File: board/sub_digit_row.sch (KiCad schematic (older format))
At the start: 86 parts, among them Q601 Q_PMOS_GSD, Q602 Q_PMOS_GSD, Q603 Q_PMOS_GSD, Q604 Q_PMOS_GSD, Q605 Q_PMOS_GSD, Q606 Q_PMOS_GSD, Q607 Q_PMOS_GSD, Q608 Q_PMOS_GSD, U601 TPIC6D595, U602 TPIC6D595, U603 TPIC6D595

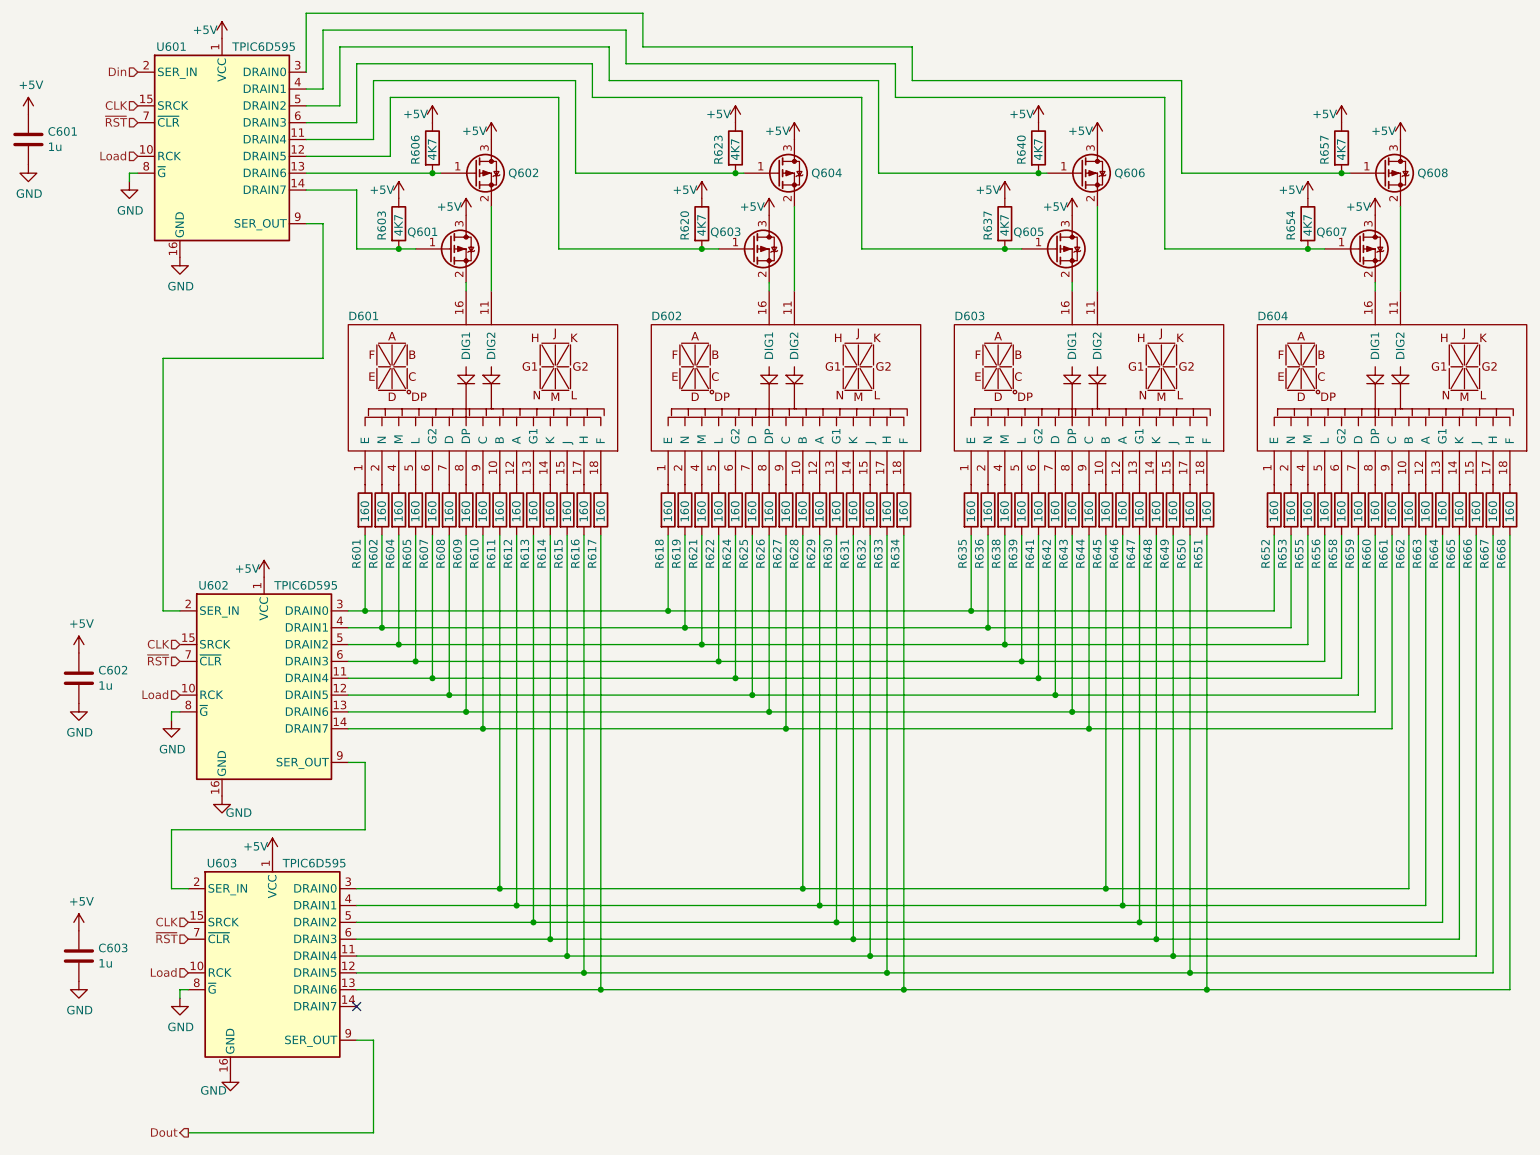
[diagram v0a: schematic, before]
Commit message: Schematics mostly complete
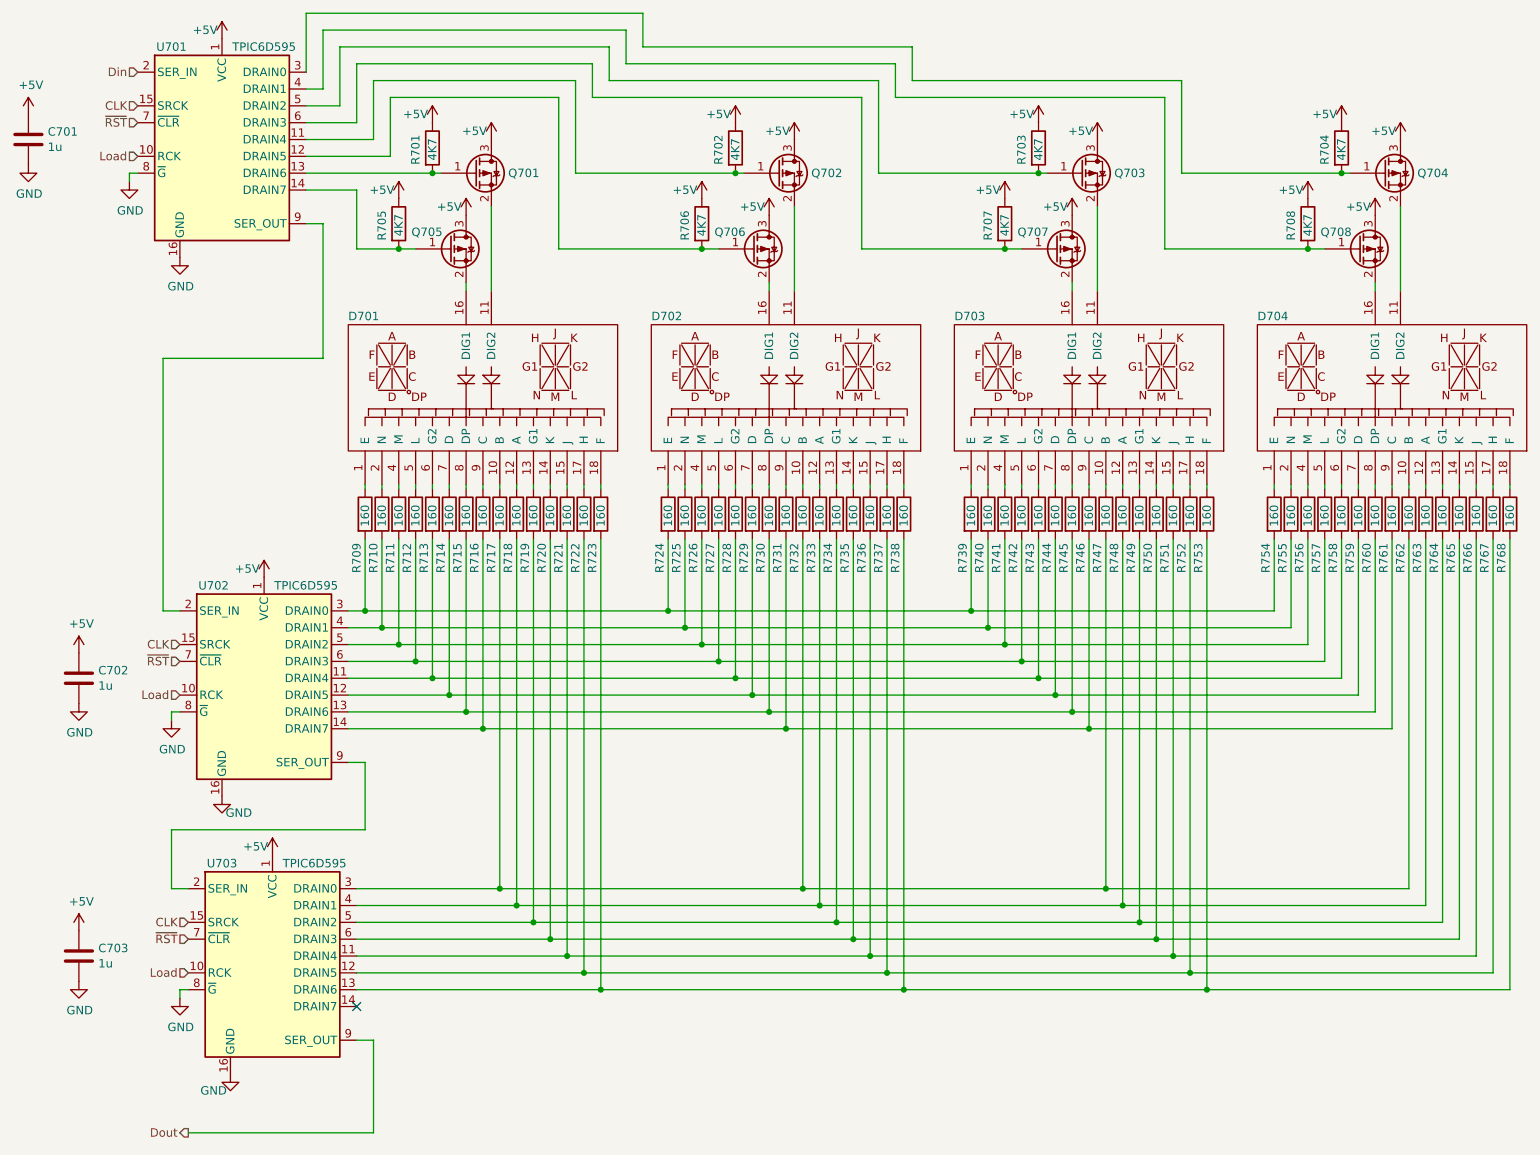
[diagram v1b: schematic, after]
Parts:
- renumbered Q602 to Q601, Q604 to Q602, Q606 to Q603, Q608 to Q604, Q601 to Q605, Q603 to Q606, Q605 to Q607, Q607 to Q608, R606 to R601, R623 to R602, R640 to R603, R657 to R604, R603 to R605, R620 to R606, R637 to R607, R654 to R608, R601 to R609, R602 to R610, R604 to R611, R605 to R612, R607 to R613, R608 to R614, R609 to R615, R610 to R616, R611 to R617, R612 to R618, R613 to R619, R614 to R620, R615 to R621, R616 to R622, R617 to R623, R618 to R624, R619 to R625, R621 to R626, R622 to R627, R624 to R628, R625 to R629, R626 to R630, R627 to R631, R628 to R632, R629 to R633, R630 to R634, R631 to R635, R632 to R636, R633 to R637, R634 to R638, R635 to R639, R636 to R640, R638 to R641, R639 to R642, R641 to R643, R642 to R644, R643 to R645, R644 to R646, R645 to R647, R646 to R648, R647 to R649, R648 to R650, R649 to R651, R650 to R652, R651 to R653, R652 to R654, R653 to R655, R655 to R656, R656 to R657
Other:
- moved on the sheet: R709, R710, R711, R712, R713, R714, R715, R716, R717, R718, R719, R720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
